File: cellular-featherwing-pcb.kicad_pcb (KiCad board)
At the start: 2 copper layers, 27 x 54 mm, 11 parts, among them J1 SIM8060-6-0-14-00-A, J2 TSM-116-01-L-SV, J3 TSM-112-01-L-SV, J4 U.FL-R-SMT(10), J5 U.FL-R-SMT(10), U1 BG96, U2 TPS63020DSJR, U3 TXB0108DQSR, U4 MAX8868EUK30+

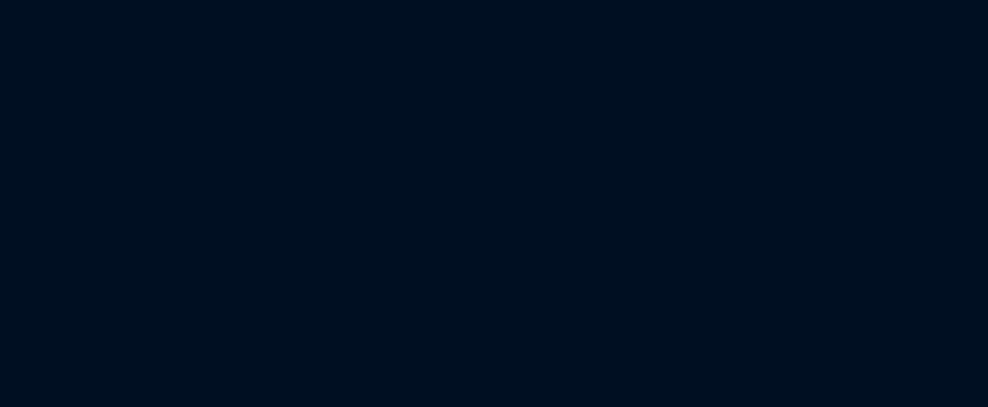
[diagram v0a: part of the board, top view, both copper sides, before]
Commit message: More progress
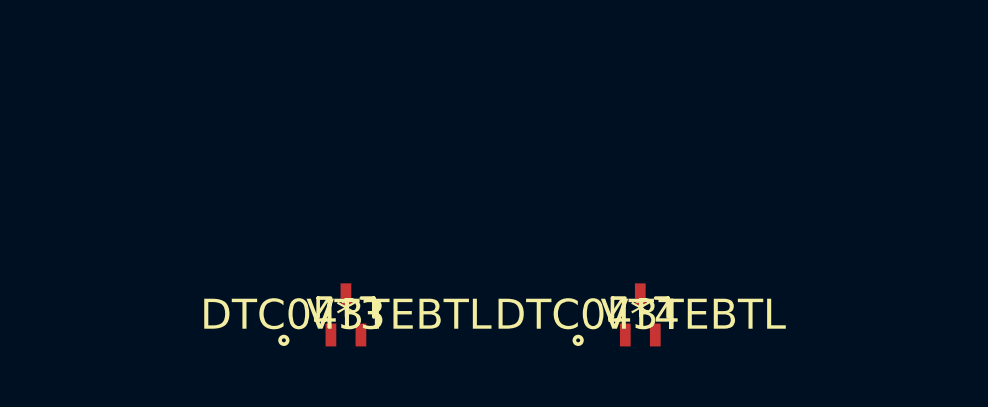
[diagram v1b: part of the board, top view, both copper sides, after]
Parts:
- added VT3: DTC043TEBTL, ul_DTC043TEBTL:DTC043TEBTL, F.Cu at (146.6, 132.7)
- added VT4: DTC043TEBTL, ul_DTC043TEBTL:DTC043TEBTL, F.Cu at (156.5, 132.7)
